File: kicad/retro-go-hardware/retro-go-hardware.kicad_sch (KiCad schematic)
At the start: 21 parts

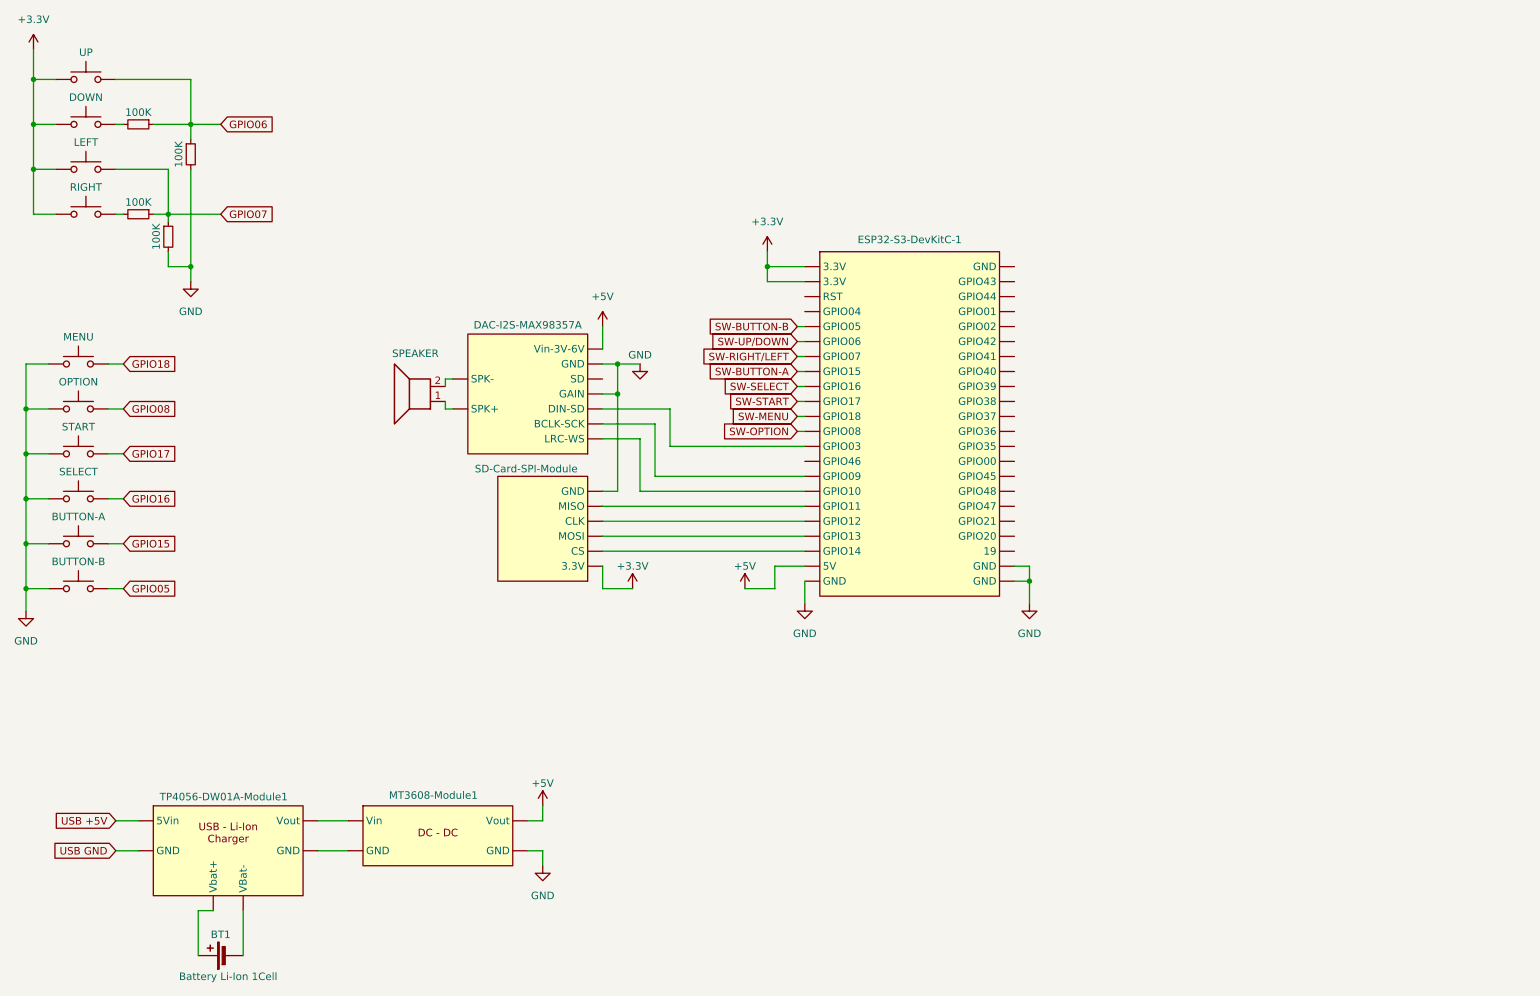
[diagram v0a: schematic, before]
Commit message: Finishing schematic
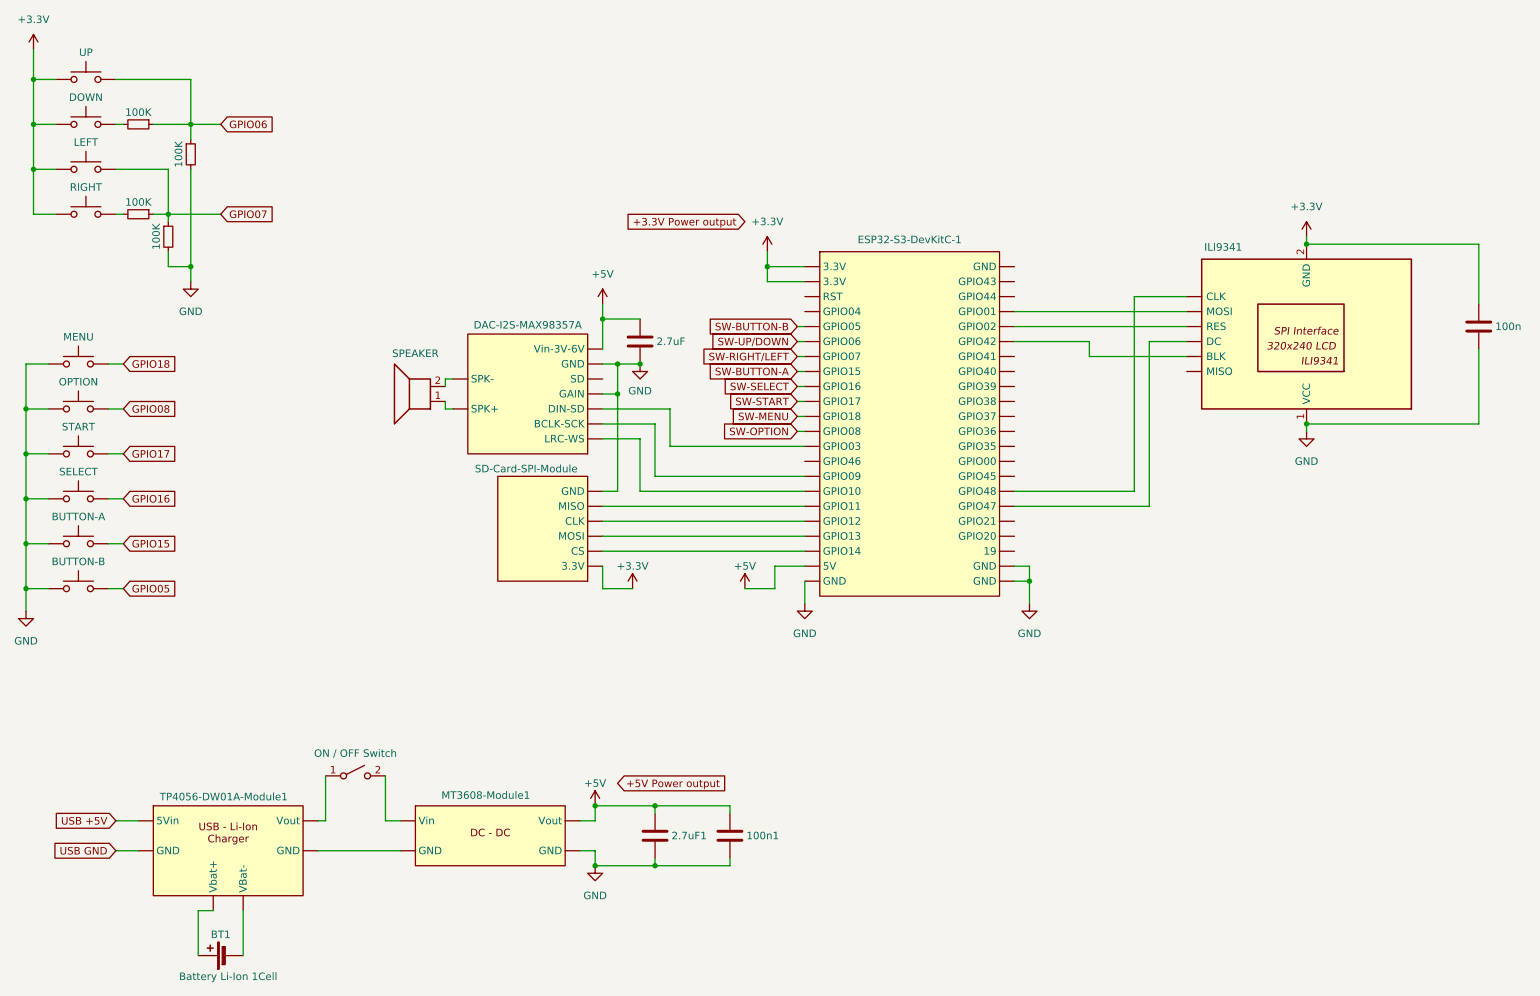
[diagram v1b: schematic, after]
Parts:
- added 100n, 100n1, 2.7uF, 2.7uF1: C, symbol Device:C
- added ILI9341: ~, symbol CustomLibrary:ILI9341-Module
- added SW1: ON / OFF Switch, symbol Switch:SW_DPST_x2
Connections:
- net +3.3V: now also 100n.1, ILI9341.2 (GND)
- net +5V: now also 100n1.1, 2.7uF.1, 2.7uF1.1
- net GND: now also 100n.2, 100n1.2, 2.7uF.2, 2.7uF1.2, ILI9341.1 (VCC)
- new net: DAC-I2S-MAX98357A. (Vin-3V-6V), ESP32-S3-DevKitC-1. (RST) (x3)
- new net: ESP32-S3-DevKitC-1. (RST), SD-Card-SPI-Module. (MOSI) (x4)
- new net: SW1.1 (A), TP4056-DW01A-Module1. (Vout)
- new net: MT3608-Module1. (Vout), SW1.2 (B)
- new net: MT3608-Module1. (Vout), TP4056-DW01A-Module1. (Vout)
- new net: ESP32-S3-DevKitC-1. (RST), ILI9341. (RES) (x5)
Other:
- moved on the sheet: MT3608-Module1
